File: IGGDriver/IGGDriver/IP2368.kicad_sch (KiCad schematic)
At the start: 23 parts, among them U16 IP2326

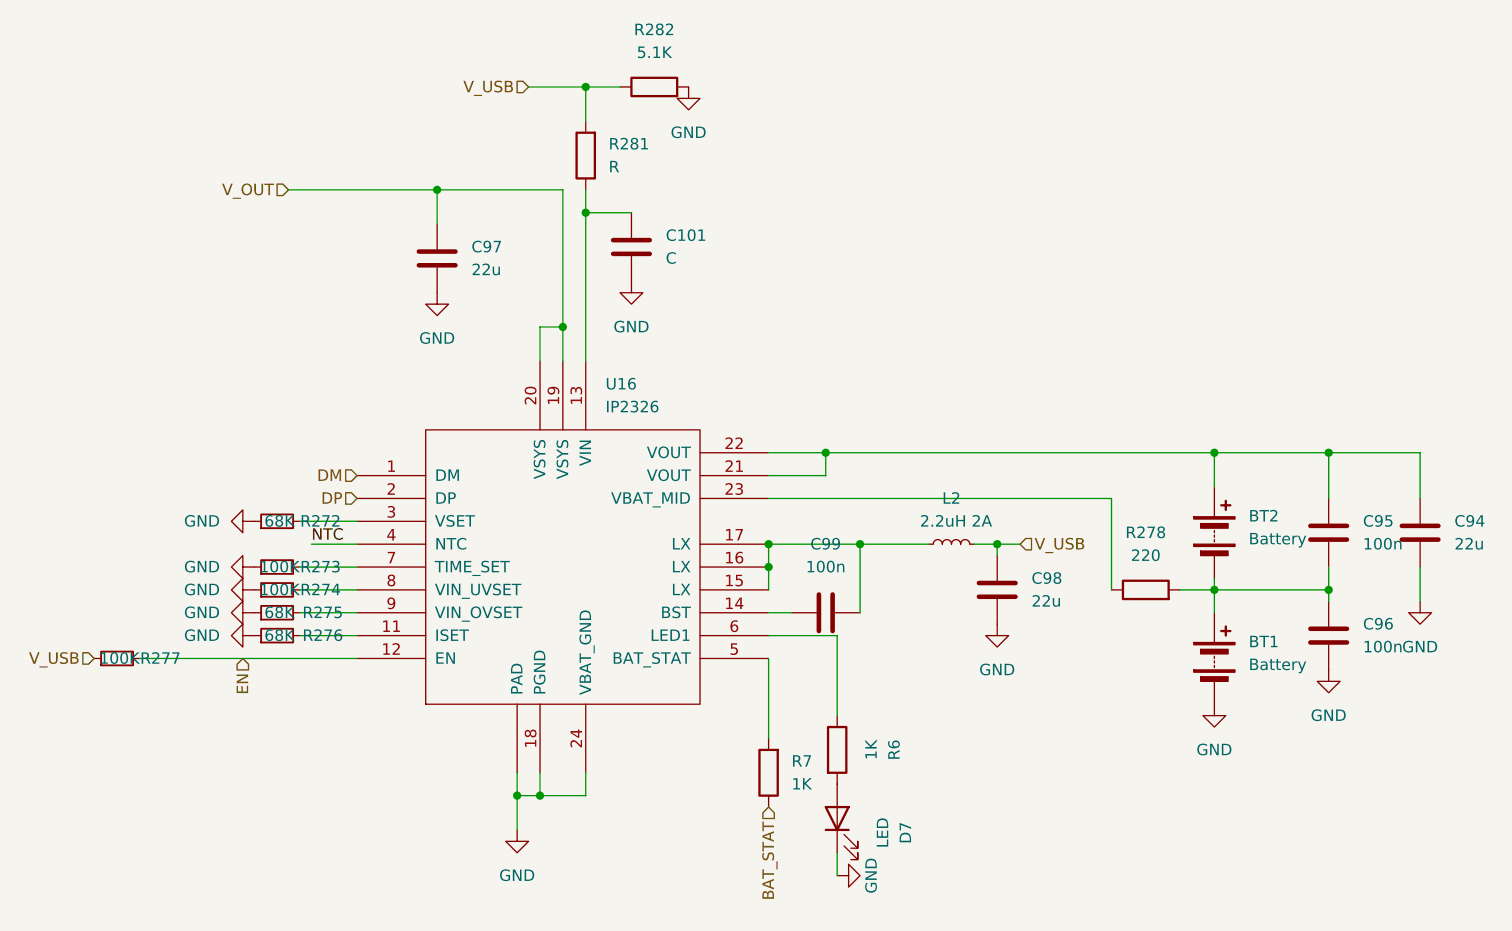
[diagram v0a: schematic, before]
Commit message: progress!
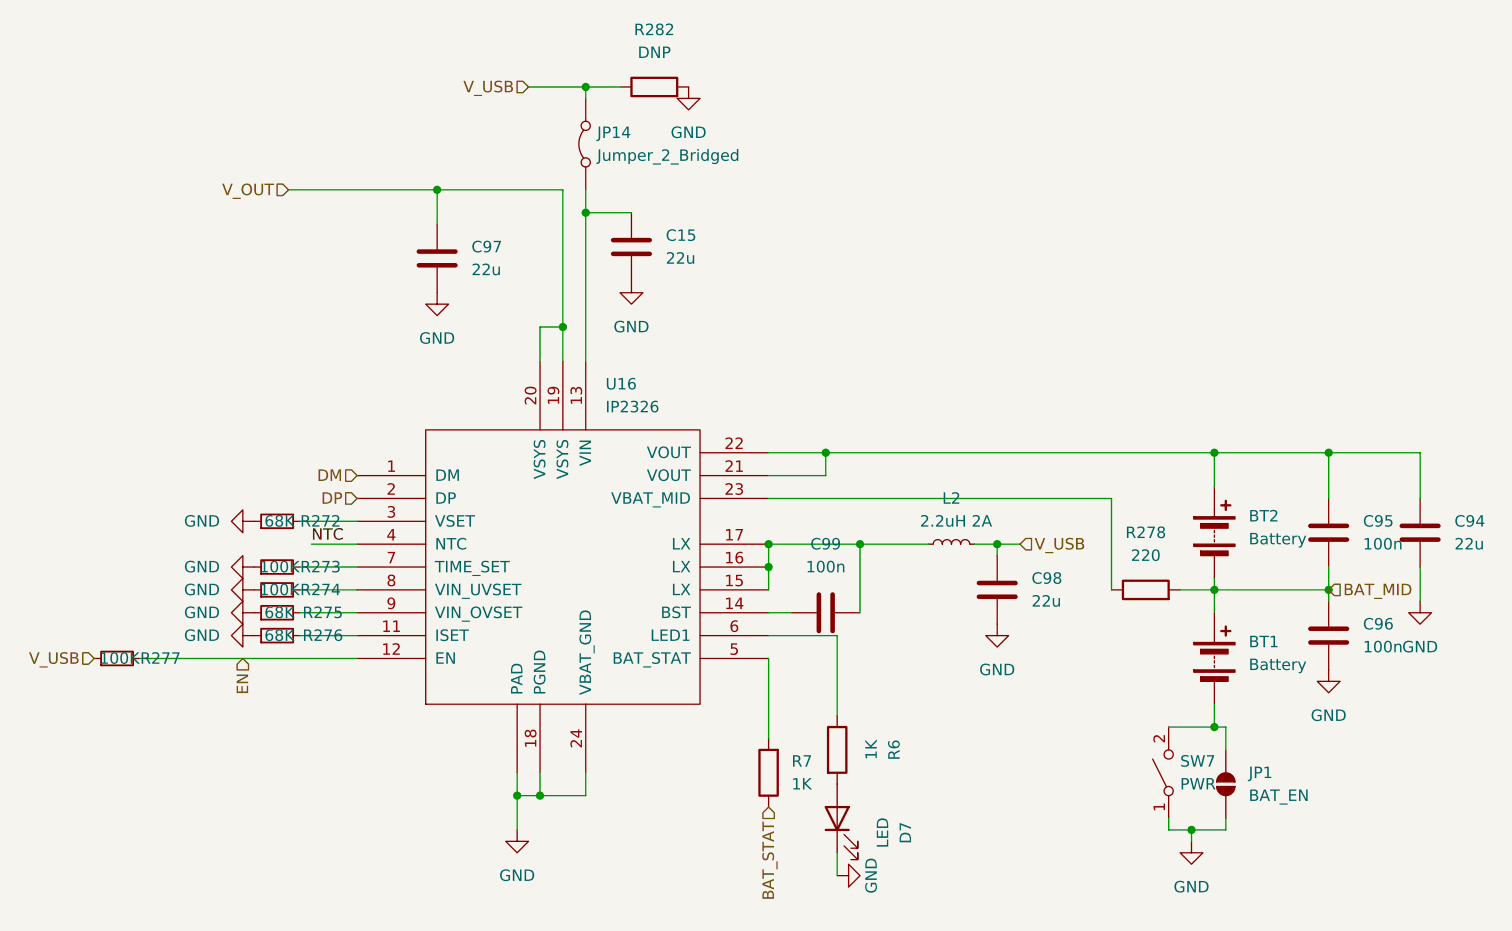
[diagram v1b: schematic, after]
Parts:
- removed C101: C, symbol Device:C
- removed R281: R, symbol Device:R
- added C15: 22u, Capacitor_SMD:C_1206_3216Metric, symbol Device:C
- added JP1: BAT_EN, symbol Jumper:SolderJumper_2_Open
- added JP14: Jumper_2_Bridged, symbol Jumper:Jumper_2_Bridged
- added SW7: PWR, symbol Switch:SW_SPST
- C95, C96, C99: footprint (none) -> Capacitor_SMD:C_0603_1608Metric; LCSC (none) -> C14663
- L2: footprint (none) -> Inductor_SMD:L_1008_2520Metric; LCSC (none) -> C488330
- R272, R275, R276: footprint (none) -> Resistor_SMD:R_0603_1608Metric; LCSC (none) -> C23231
- R273, R274, R277: footprint (none) -> Resistor_SMD:R_0603_1608Metric; LCSC (none) -> C25803
- R278: footprint (none) -> Resistor_SMD:R_0603_1608Metric; LCSC (none) -> C22962
- R282: value 5.1K -> DNP; footprint (none) -> Resistor_SMD:R_0603_1608Metric
- U16: footprint MODULE -> Package_DFN_QFN:QFN-24-1EP_4x4mm_P0.5mm_EP2.6x2.6mm_ThermalVias; LCSC (none) -> C2832094
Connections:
- net GND: now also C15.2, JP1.1 (A), SW7.1 (A); no longer BT1.2 (-)
- net V_USB: now also JP14.2 (B)
- net at U16.13 (VIN): now also C15.1, JP14.1 (A)
- net BAT_MID: now reaches BT1.1 (+), BT2.2 (-), C95.2, C96.1, R278.2
- new net: BT1.2 (-), JP1.2 (B), SW7.2 (B)
